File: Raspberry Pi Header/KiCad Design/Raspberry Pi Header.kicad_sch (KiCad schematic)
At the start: 1 part, among them J1 Raspberry Pi Header

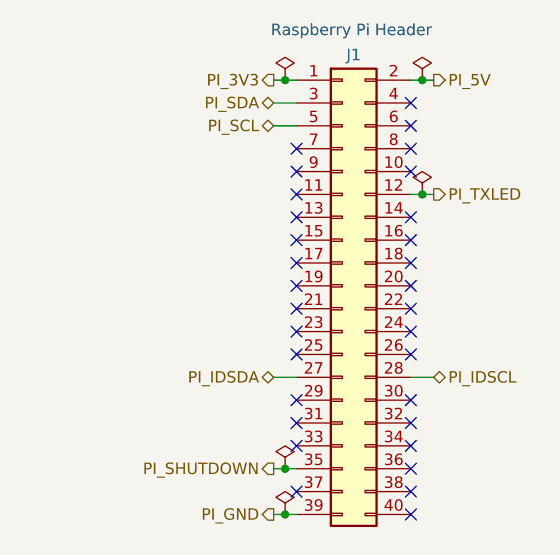
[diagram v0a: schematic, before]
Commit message: Notionally complete through PA
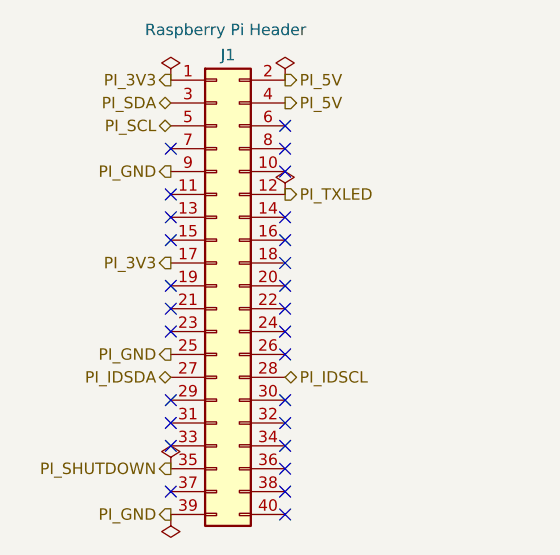
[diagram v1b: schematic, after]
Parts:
- J1: footprint (none) -> Wsprry Pi µHAT+:PinSocket_2x20_P2.54mm_Vertical
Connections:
- net PI_3V3: now also J1.17 (3V3)
- net PI_5V: now also J1.4 (5V)
- net PI_GND: now also J1.25 (GND), J1.9 (GND)
- no-connect marks 31 -> 27
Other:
- company: (none) -> Lee C. Bussy [AA0NT]
- title: (none) -> Raspberry Pi Header
- moved on the sheet: J1
